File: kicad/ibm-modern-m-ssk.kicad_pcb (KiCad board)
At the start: 2 copper layers, 100 x 50 mm, 50 parts, among them J1 TF38-24S-0.5SV(830), J2 S2B-PH-SM4-TB(LF)(SN), J4 Conn_01x04_Pin, J5 726386-2, Q1 DMP2123LQ, SW90 SW_Push, U1 NRF52840, U2 nPM1300-QEAA, Y1 32MHz, Y2 32.768 kHz

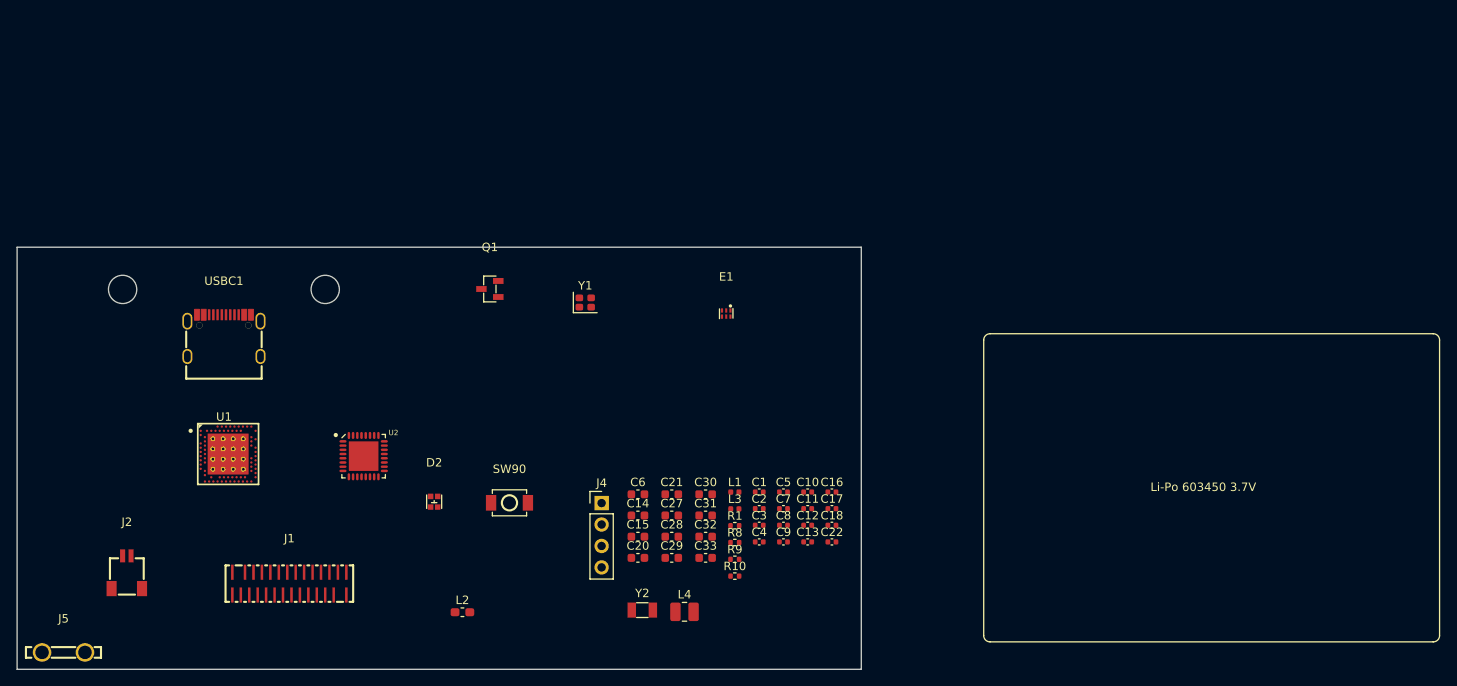
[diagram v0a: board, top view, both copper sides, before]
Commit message: update - pcb layout
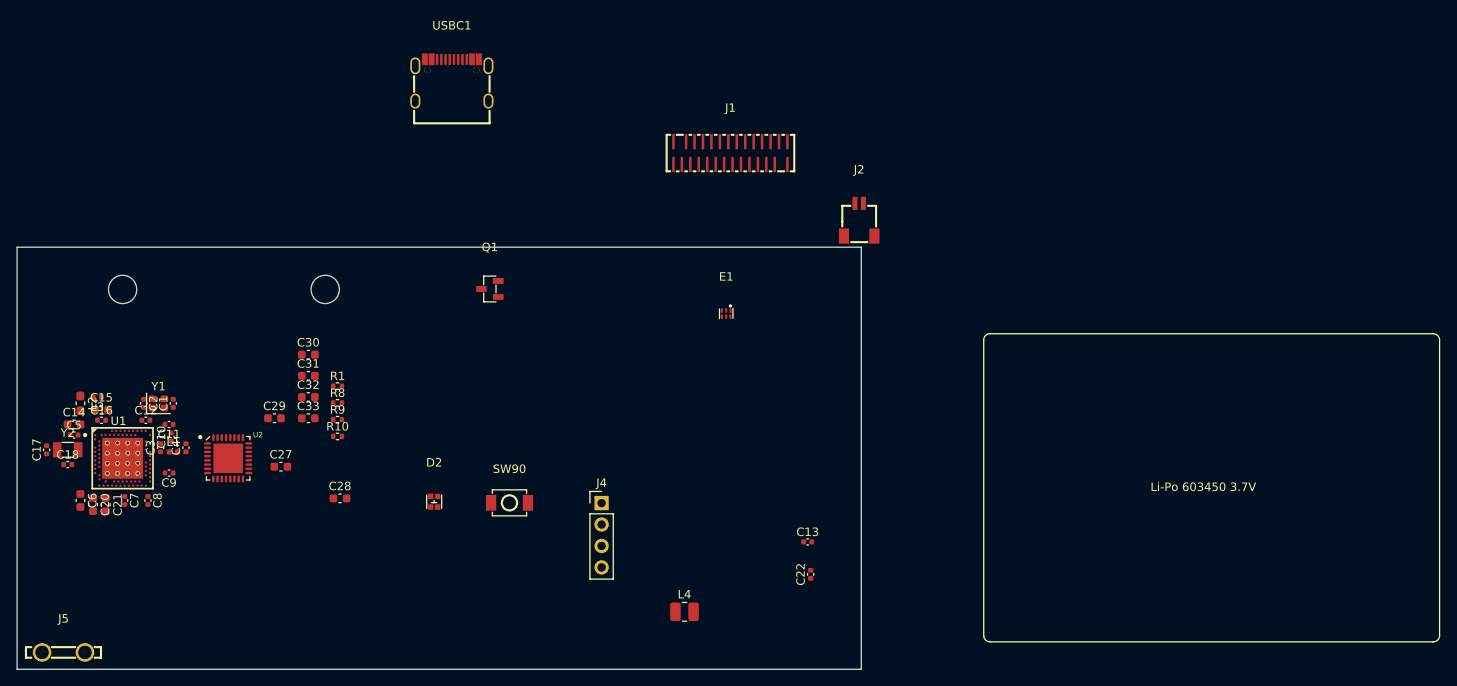
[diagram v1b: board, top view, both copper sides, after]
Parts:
- moved J2 96.3 mm to (149.8, 46.8)
- moved C17 93.3 mm to (53.5, 74.0), turned to 90 degrees
- moved C18 90.8 mm to (56.0, 75.8)
- moved C16 86.9 mm to (60.0, 70.5)
- moved C5 84.3 mm to (56.8, 72.2)
- moved C12 79.4 mm to (65.2, 70.5)
- moved C7 78.0 mm to (62.8, 80.0), turned to -90 degrees
- moved L3 76.7 mm to (59.5, 67.8), turned to 180 degrees
- moved C11 76.3 mm to (68.0, 71.0), turned to 180 degrees
- moved C10 75.7 mm to (68.2, 72.5), turned to 90 degrees
- moved C8 75.3 mm to (65.5, 80.0), turned to -90 degrees
- moved C2 74.0 mm to (65.0, 68.5), turned to -90 degrees
- moved C9 73.2 mm to (68.0, 76.8), turned to 180 degrees
- moved J1 73.0 mm to (134.5, 38.9)
- moved C3 71.5 mm to (67.0, 73.8), turned to 90 degrees
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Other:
- copper layers 2 -> 4
